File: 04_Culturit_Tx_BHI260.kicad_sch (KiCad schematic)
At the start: 1 part, among them U15 BHI260AP

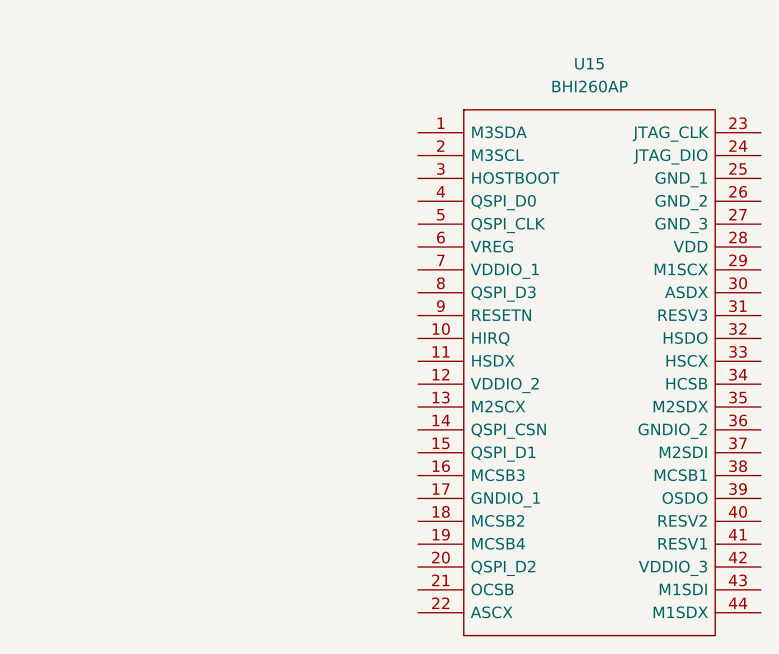
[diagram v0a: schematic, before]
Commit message: 2022-08-09
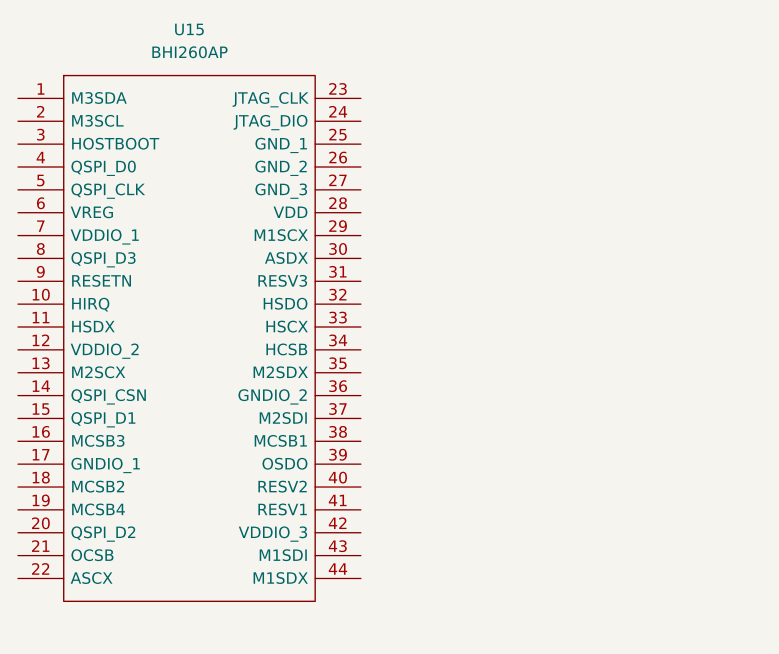
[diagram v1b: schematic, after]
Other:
- moved on the sheet: U15
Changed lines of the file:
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@@
 (kicad_sch (version 20211123) (generator eeschema)
   (paper "A4")
-  (symbol (lib_id "BHI260AP:BHI260AP") (at 139.7 72.39 0) (unit 1)
+  (symbol (lib_id "BHI260AP:BHI260AP") (at 95.25 68.58 0) (unit 1)
     (in_bom yes) (on_board yes) (fields_autoplaced)
-    (property "Reference" "U15" (id 0) (at 158.75 64.77 0))
-    (property "Value" "BHI260AP" (id 1) (at 158.75 67.31 0))
-    (property "Footprint" "Local_devices:BHI260AP" (id 2) (at 173.99 69.85 0)
+    (property "Reference" "U15" (id 0) (at 114.3 60.96 0))
+    (property "Value" "BHI260AP" (id 1) (at 114.3 63.5 0))
+    (property "Footprint" "Local_devices:BHI260AP" (id 2) (at 129.54 66.04 0)
       (effects (font (size 1.27 1.27)) (justify left) hide)
     )
-    (property "Datasheet" "https://www.bosch-sensortec.com/media/boschsensortec/downloads/datasheets/bst-bhi260ap-ds000.pdf" (id 3) (at 173.99 72.39 0)
+    (property "Datasheet" "https://www.bosch-sensortec.com/media/boschsensortec/downloads/datasheets/bst-bhi260ap-ds000.pdf" (id 3) (at 129.54 68.58 0)
       (effects (font (size 1.27 1.27)) (justify left) hide)
     )
-    (property "Description" "Multiple Function Sensor Modules Self-Learning AI sensor with integrated microcontroller and an IMU" (id 4) (at 173.99 74.93 0)
+    (property "Description" "Multiple Function Sensor Modules Self-Learning AI sensor with integrated microcontroller and an IMU" (id 4) (at 129.54 71.12 0)
       (effects (font (size 1.27 1.27)) (justify left) hide)
     )
-    (property "Height" "0.87" (id 5) (at 173.99 77.47 0)
+    (property "Height" "0.87" (id 5) (at 129.54 73.66 0)
       (effects (font (size 1.27 1.27)) (justify left) hide)
     )
-    (property "Mouser Part Number" "262-BHI260AP" (id 6) (at 173.99 80.01 0)
+    (property "Mouser Part Number" "262-BHI260AP" (id 6) (at 129.54 76.2 0)
       (effects (font (size 1.27 1.27)) (justify left) hide)
     )
-    (property "Mouser Price/Stock" "https://www.mouser.co.uk/ProductDetail/Bosch-Sensortec/BHI260AP?qs=T94vaHKWudTEPTnGI%252BTy9w%3D%3D" (id 7) (at 173.99 82.55 0)
+    (property "Mouser Price/Stock" "https://www.mouser.co.uk/ProductDetail/Bosch-Sensortec/BHI260AP?qs=T94vaHKWudTEPTnGI%252BTy9w%3D%3D" (id 7) (at 129.54 78.74 0)
       (effects (font (size 1.27 1.27)) (justify left) hide)
     )
-    (property "Manufacturer_Name" "Bosch Sensortec" (id 8) (at 173.99 85.09 0)
+    (property "Manufacturer_Name" "Bosch Sensortec" (id 8) (at 129.54 81.28 0)
       (effects (font (size 1.27 1.27)) (justify left) hide)
     )
-    (property "Manufacturer_Part_Number" "BHI260AP" (id 9) (at 173.99 87.63 0)
+    (property "Manufacturer_Part_Number" "BHI260AP" (id 9) (at 129.54 83.82 0)
       (effects (font (size 1.27 1.27)) (justify left) hide)
     )
